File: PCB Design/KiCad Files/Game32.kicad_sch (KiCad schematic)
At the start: 20 parts, among them SW1 UP, SW2 DOWN, SW3 LEFT, SW4 RIGHT, SW5 SELECT, SW6 START, SW7 A, SW8 KEY, SW9 B, U1 ESP32-WROOM-32

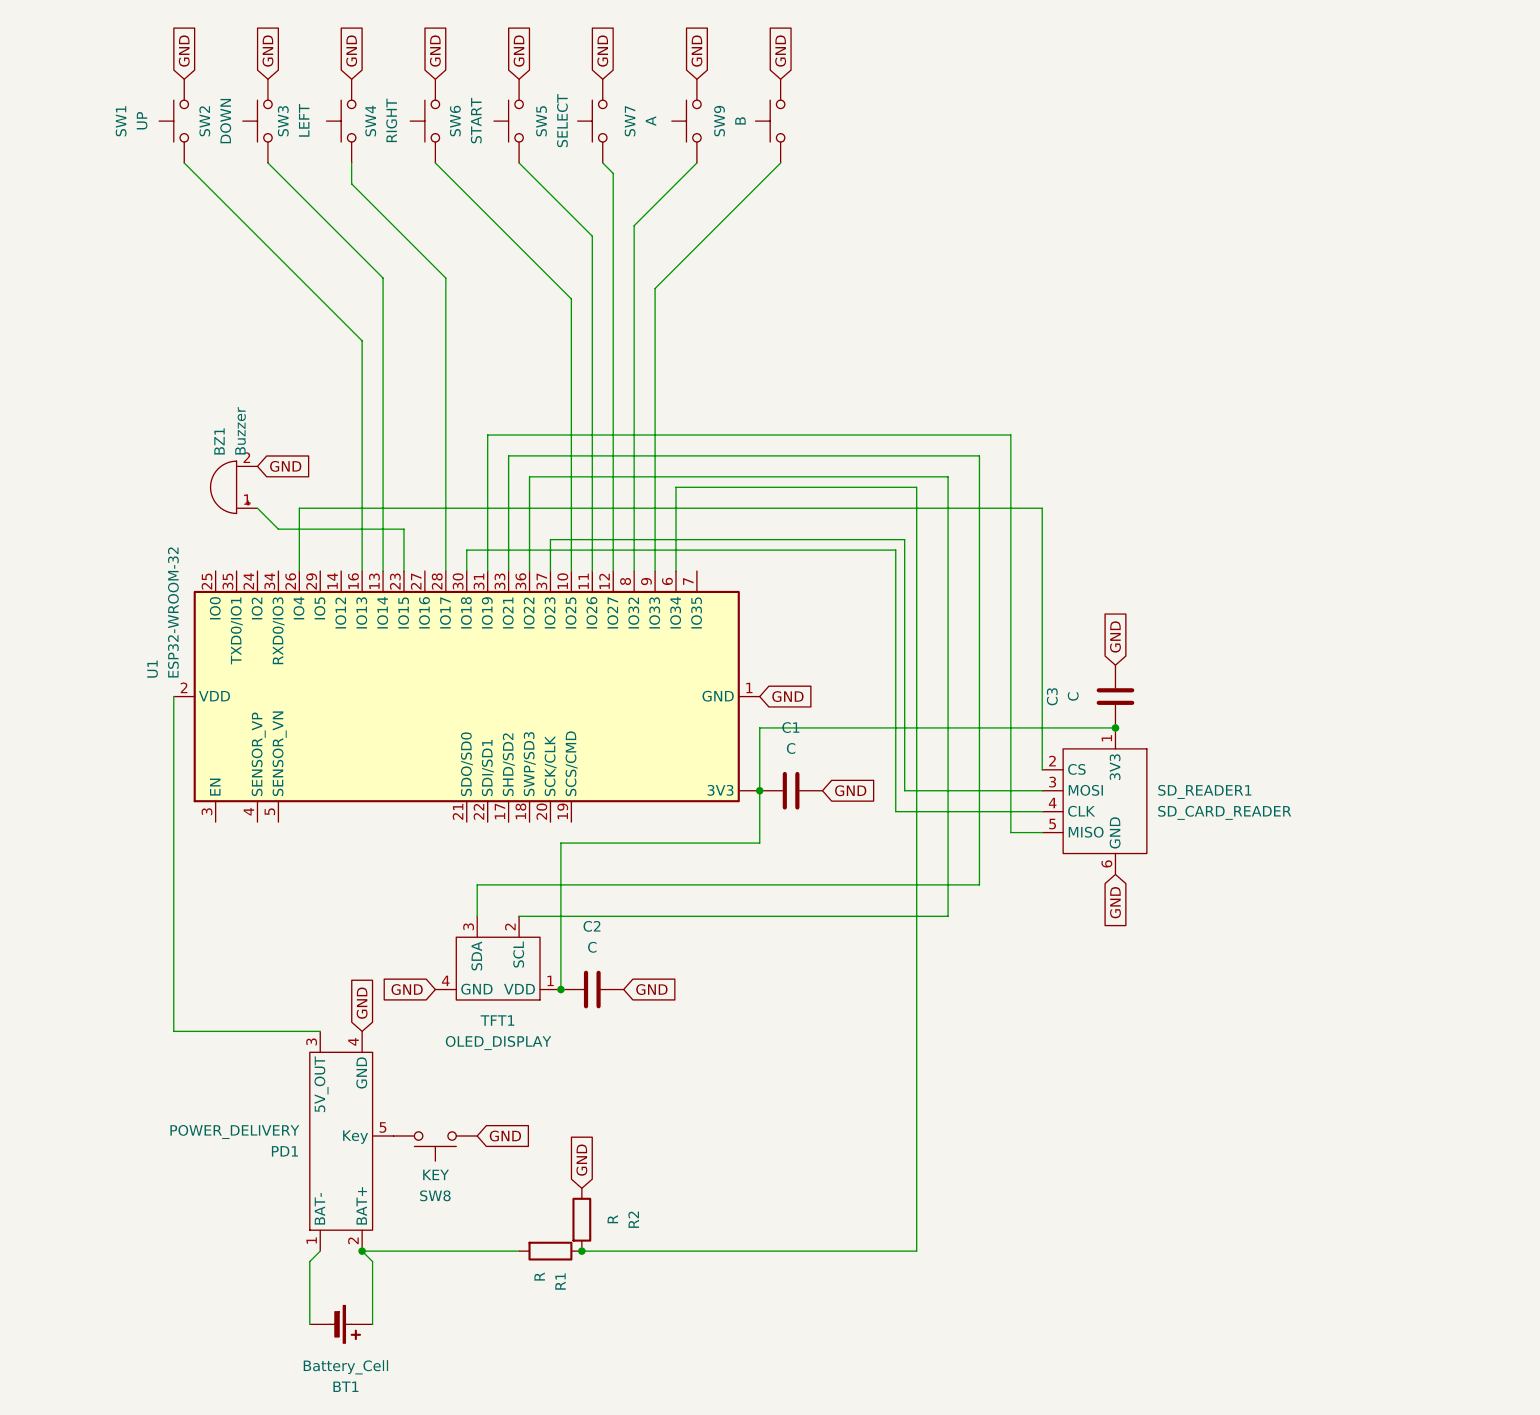
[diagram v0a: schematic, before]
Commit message: PCB Completed
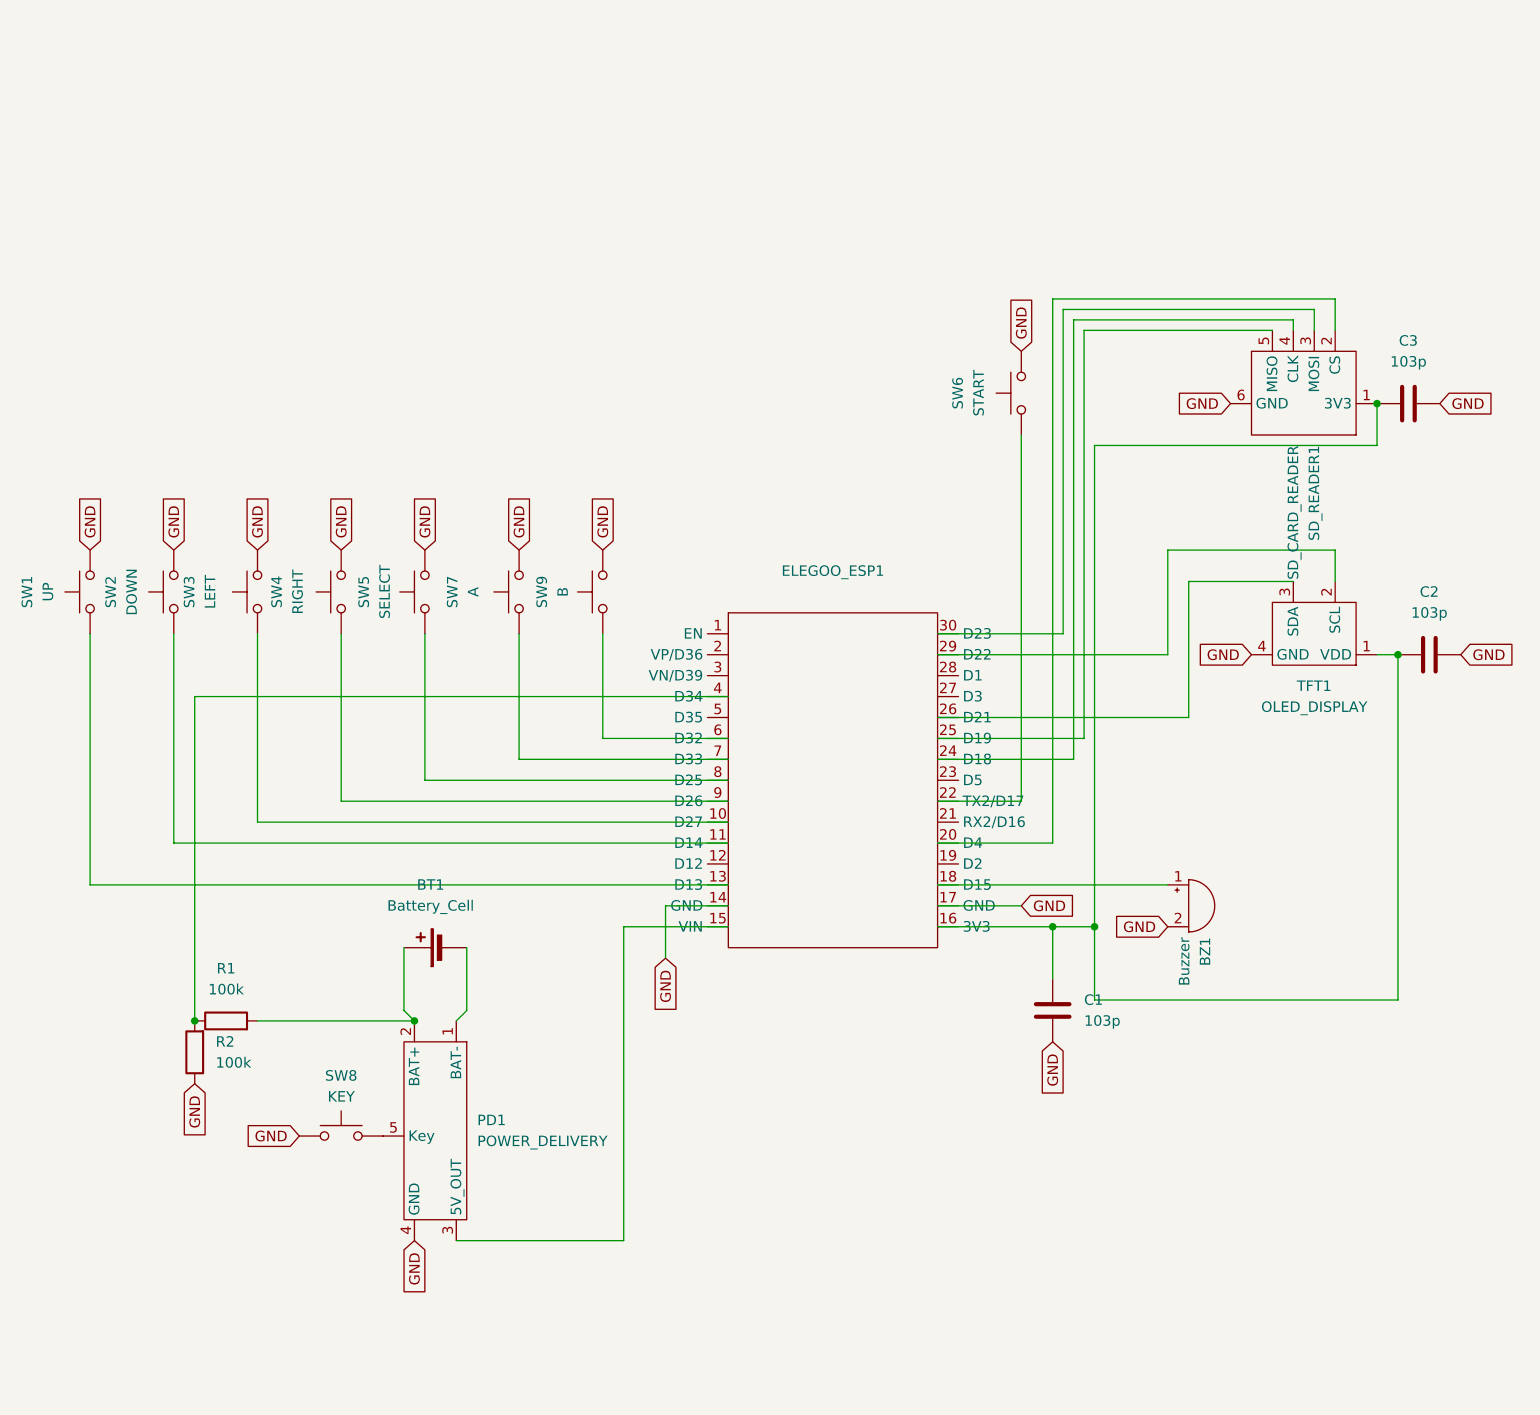
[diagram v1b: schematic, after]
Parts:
- removed U1: ESP32-WROOM-32, RF_Module:ESP32-C3-DevKit-ELEGOO, symbol RF_Module:ESP32-WROOM-32
- added ELEGOO_ESP1: ~, Custom Devkits:ELEGOO ESP32 DevKit Type C V1, symbol Custom Devkits:ELEGOO_ESP32_DevKit_Type_C_V1
- BT1, BZ1, PD1, SD_READER1, SW1, SW2, SW3, SW4, SW5, SW6, SW7, SW8, SW9, TFT1: now left out of the parts list
- C1, C2, C3: value C -> 103p; LCSC (none) -> C1710
- R1, R2: value R -> 100k; LCSC (none) -> C149504
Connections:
- net GND: now also C1.1, ELEGOO_ESP1.14 (GND), ELEGOO_ESP1.17 (GND); no longer C1.2
- net at BZ1.1 (+): now also ELEGOO_ESP1.18 (D15)
- net at SW2.1: now also ELEGOO_ESP1.11 (D14)
- net at SW6.1: now also ELEGOO_ESP1.22 (TX2/D17)
- net at SW7.1: now also ELEGOO_ESP1.7 (D33)
- net at SW1.1: now also ELEGOO_ESP1.13 (D13)
- net at R1.1, R2.2: now also ELEGOO_ESP1.4 (D34)
- net at SW5.1: now also ELEGOO_ESP1.8 (D25)
- net at C2.1, C3.1, SD_READER1.1 (3V3)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: now also C1.2, ELEGOO_ESP1.16 (3V3); no longer C1.1
- net at TFT1.2 (SCL): now also ELEGOO_ESP1.29 (D22)
- net at TFT1.3 (SDA): now also ELEGOO_ESP1.26 (D21)
- net at SD_READER1.2 (CS): now also ELEGOO_ESP1.20 (D4)
- net at SD_READER1.3 (MOSI): now also ELEGOO_ESP1.30 (D23)
- net at SD_READER1.4 (CLK): now also ELEGOO_ESP1.24 (D18)
- net at SD_READER1.5 (MISO): now also ELEGOO_ESP1.25 (D19)
- net at SW3.1: now also ELEGOO_ESP1.10 (D27)
- net at SW9.1: now also ELEGOO_ESP1.6 (D32)
- net at SW4.1: now also ELEGOO_ESP1.9 (D26)
- net at PD1.3 (5V_OUT): now also ELEGOO_ESP1.15 (VIN)
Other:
- moved on the sheet: BT1, BZ1, C2, C3, PD1, R1, R2, SD_READER1, SW1, SW2, SW3, SW4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
